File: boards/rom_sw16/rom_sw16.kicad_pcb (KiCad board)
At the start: 2 copper layers, 99.1 x 99.1 mm, 103 parts, among them J1 Conn_02x10_Top_Bottom, SW1 SW_DIP_x08, SW10 SW_DIP_x08, SW11 SW_DIP_x08, SW12 SW_DIP_x08, SW13 SW_DIP_x08, SW14 SW_DIP_x08, SW15 SW_DIP_x08, SW16 SW_DIP_x08, SW2 SW_DIP_x08, SW3 SW_DIP_x08, SW4 SW_DIP_x08, SW5 SW_DIP_x08, SW6 SW_DIP_x08, SW7 SW_DIP_x08, SW8 SW_DIP_x08, SW9 SW_DIP_x08, U1 74HC138, U2 74HC158, U3 74HC158

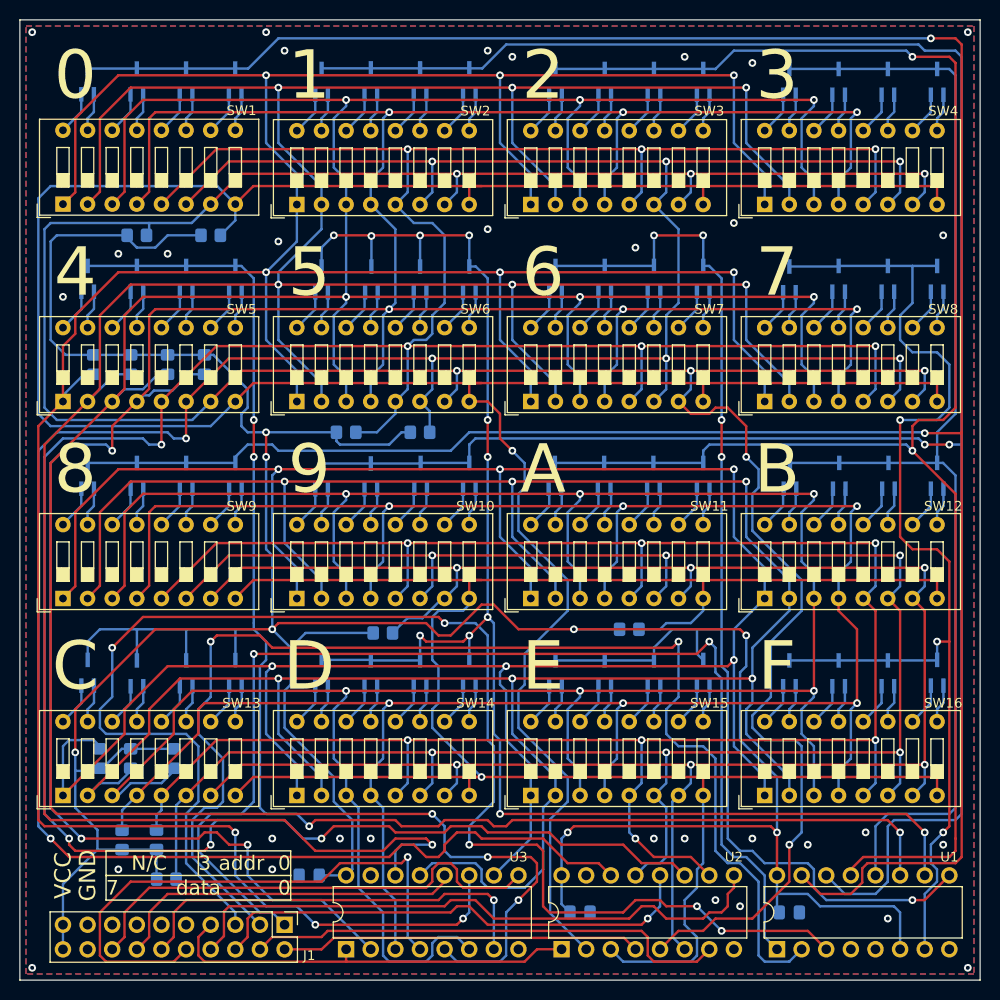
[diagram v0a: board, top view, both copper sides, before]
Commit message: unify libraries
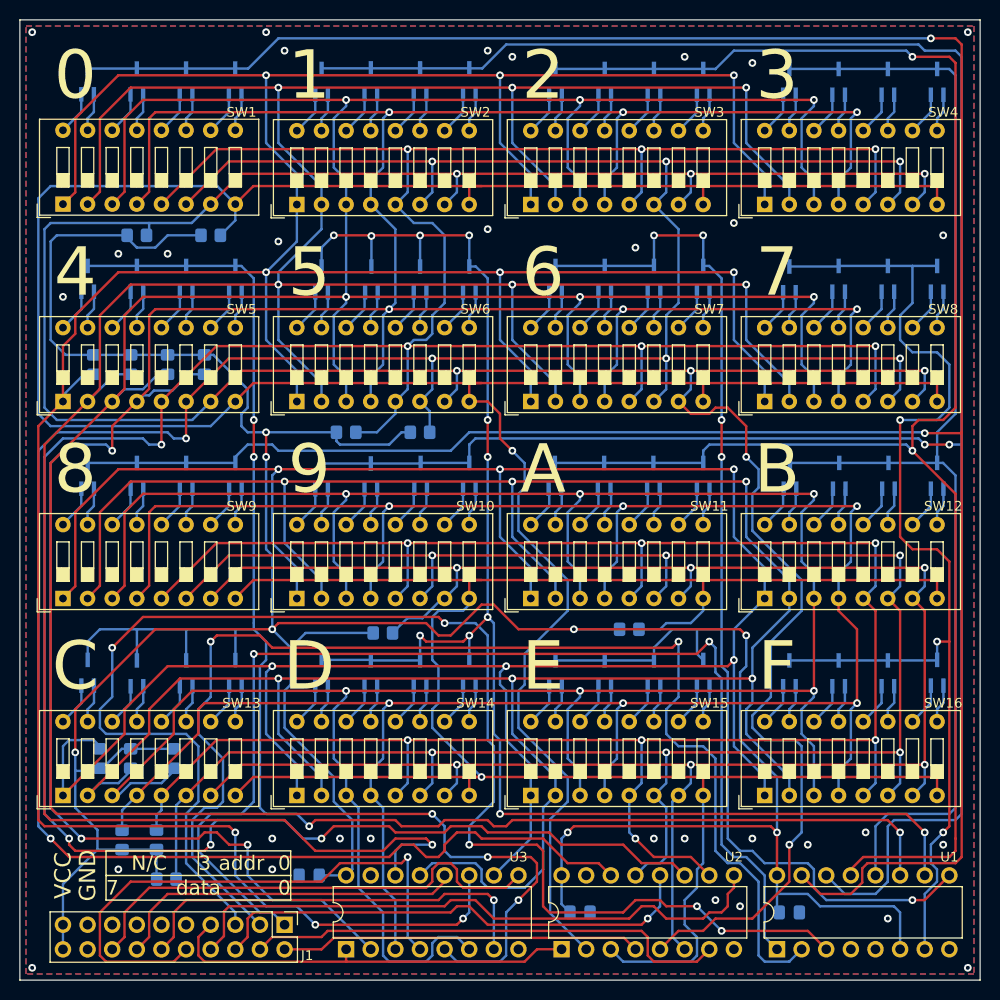
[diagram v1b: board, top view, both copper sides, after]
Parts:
- J1: footprint PrjLibrary_MainBoard:PinHeader_2x10_P2.54mm_Vertical_Top_Bottom -> ModifiedKiCadLibrary:PinHeader_2x10_P2.54mm_Vertical_Top_Bottom
- SW1, SW10, SW11, SW12, SW13, SW14, SW15, SW16, SW2, SW3, SW4, SW5, SW6, SW7, SW8, SW9: footprint PrjLibrary:SW_DIP_SPSTx08_Slide_9.78x22.5mm_W7.62mm_P2.54mm_3Dfixed -> ModifiedKiCadLibrary:SW_DIP_SPSTx08_Slide_9.78x22.5mm_W7.62mm_P2.54mm_3Dfixed
- U1, U2, U3: footprint PrjLibrary_MainBoard:DIP-16_W7.62mm_D1mm -> ModifiedKiCadLibrary:DIP-16_W7.62mm_D1mm
